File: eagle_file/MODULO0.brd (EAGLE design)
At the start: 89.8 x 69.8 mm, 3 parts

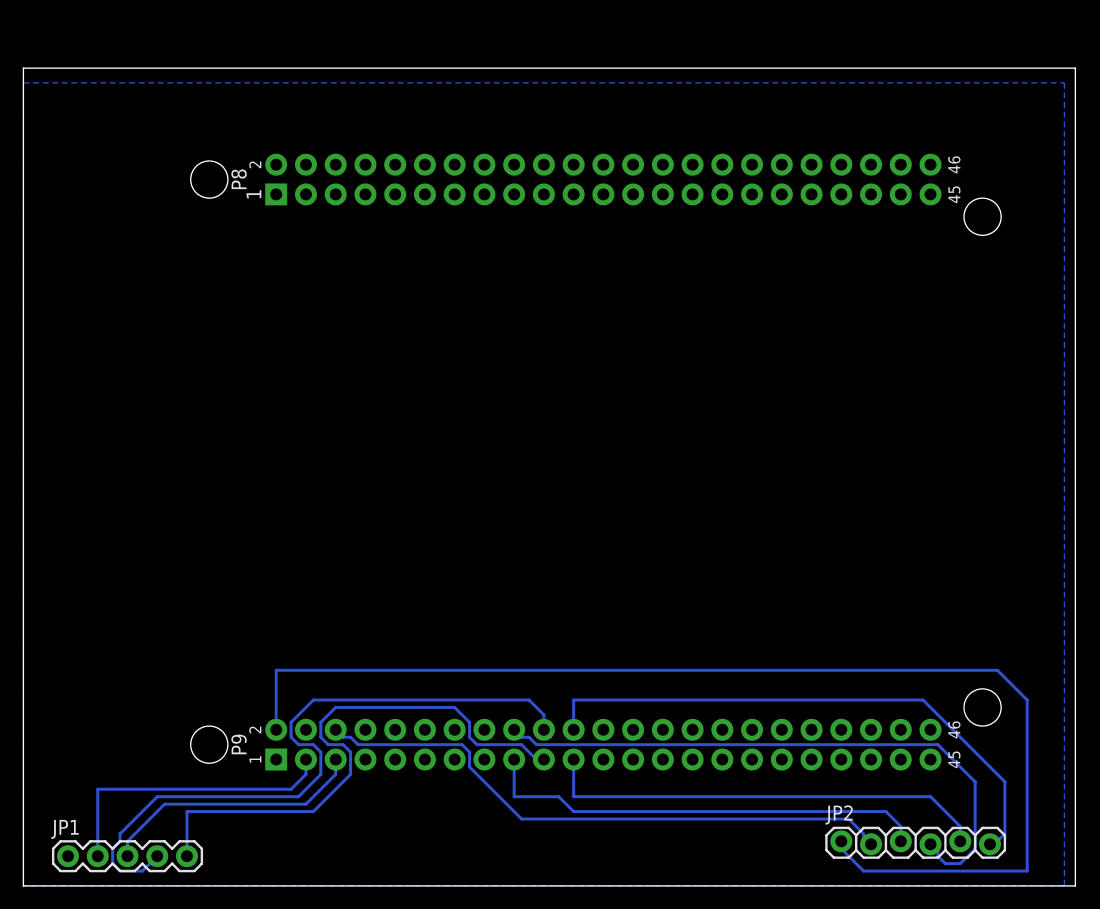
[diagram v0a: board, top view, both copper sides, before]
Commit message: Modulo1
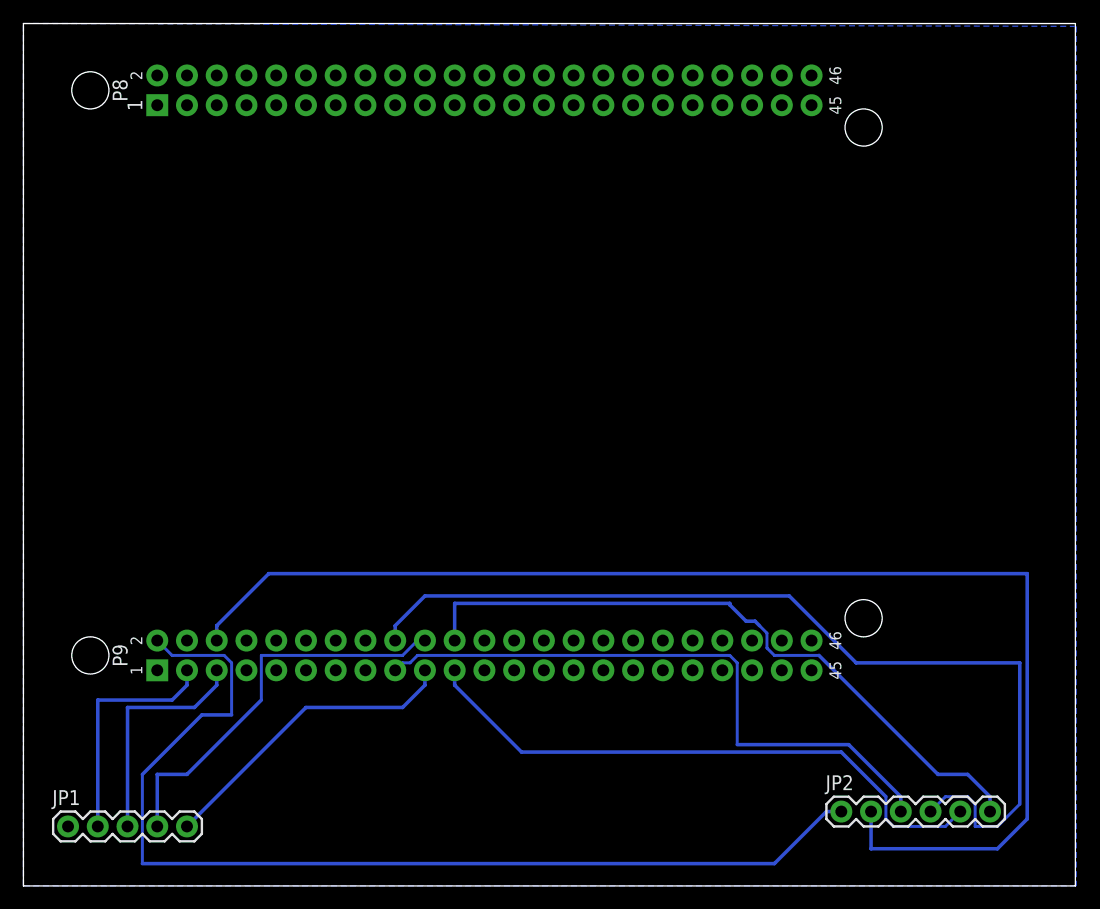
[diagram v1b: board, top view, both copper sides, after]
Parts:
- JP2: device SparkFun-Connectors:1X06_LOCK -> SparkFun-Connectors:1X06
- moved U$1 12.7 mm to (-8.89, 16.5)
- moved JP1 2.54 mm to (3.81, 5.08)
- moved JP2 2.54 mm to (69.8, 6.35)
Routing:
- net N$7: track 51.0 -> 110.8 mm
- net N$9: track 52.5 -> 81.2 mm
- net N$5: track 57.1 -> 34.3 mm
- net N$4: track 47.5 -> 26.6 mm
- net N$8: track 38.5 -> 54.1 mm
- net N$11: track 38.5 -> 51.1 mm
- net N$6: track 102.2 -> 90.5 mm
- net N$10: track 48.5 -> 57.8 mm
- net N$2: track 25.3 -> 20.2 mm
- net N$3: track 22.7 -> 19.8 mm
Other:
- board size 89.8 x 69.8 mm -> 89.8 x 73.7 mm
